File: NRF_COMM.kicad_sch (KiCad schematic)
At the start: 2 parts, among them U5 NRF24L01_Breakout

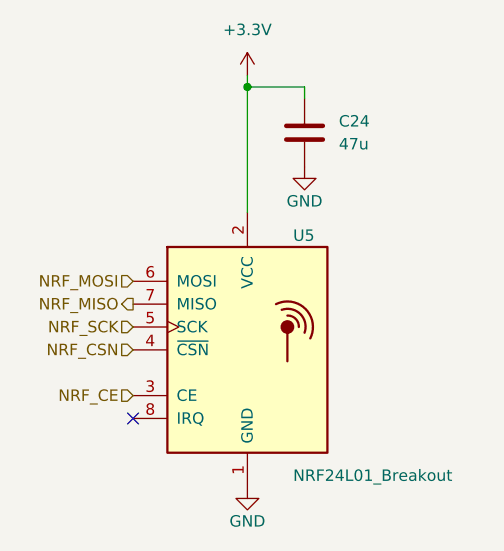
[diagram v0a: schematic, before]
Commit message: changed pins
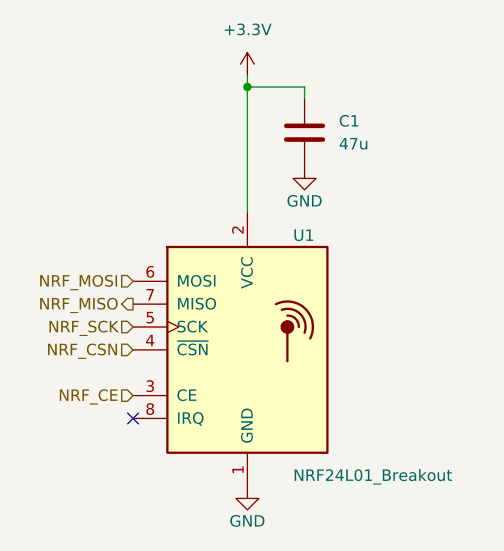
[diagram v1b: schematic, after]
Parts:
- C1: renamed from C24; footprint Capacitor_THT:CP_Radial_D5.0mm_P2.00mm -> Capacitor_THT:CP_Radial_D4.0mm_P1.50mm
- renumbered U5 to U1
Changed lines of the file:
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@@
   (symbol (lib_id "RF:NRF24L01_Breakout") (at 139.7 100.33 0) (unit 1)
     (in_bom yes) (on_board yes) (dnp no)
-    (property "Reference" "U5" (at 144.78 87.63 0)
+    (property "Reference" "U1" (at 144.78 87.63 0)
       (effects (font (size 1.27 1.27)) (justify left))
     )
@@
       (project "electrium-esc-v2"
         (path "/be00c12c-11fa-42cb-8a0b-46fcd24b2ced/81cbbca5-64b8-44af-87f0-aec946520ae6"
-          (reference "U5") (unit 1)
+          (reference "U1") (unit 1)
         )
       )
       (project "electrium-esc"
         (path "/d277d506-2f4d-497b-a498-1ff059e212d2/9d2b8e53-abda-48f4-a6e0-4b62c24d8218"
-          (reference "U?") (unit 1)
+          (reference "U5") (unit 1)
         )
       )
@@
   (symbol (lib_id "power:GND") (at 146.05 80.01 0) (unit 1)
     (in_bom yes) (on_board yes) (dnp no)
-    (property "Reference" "#PWR037" (at 146.05 86.36 0)
+    (property "Reference" "#PWR03" (at 146.05 86.36 0)
       (effects (font (size 1.27 1.27)) hide)
     )
@@
       (project "electrium-esc-v2"
         (path "/be00c12c-11fa-42cb-8a0b-46fcd24b2ced/81cbbca5-64b8-44af-87f0-aec946520ae6"
-          (reference "#PWR037") (unit 1)
+          (reference "#PWR03") (unit 1)
         )
       )
       (project "electrium-esc"
         (path "/d277d506-2f4d-497b-a498-1ff059e212d2/9d2b8e53-abda-48f4-a6e0-4b62c24d8218"
-          (reference "#PWR?") (unit 1)
+          (reference "#PWR072") (unit 1)
         )
       )
@@
   (symbol (lib_id "Device:C") (at 146.05 76.2 0) (unit 1)
     (in_bom yes) (on_board yes) (dnp no) (fields_autoplaced)
-    (property "Reference" "C24" (at 149.86 74.9299 0)
+    (property "Reference" "C1" (at 149.86 74.9299 0)
       (effects (font (size 1.27 1.27)) (justify left))
     )
@@
       (effects (font (size 1.27 1.27)) (justify left))
     )
-    (property "Footprint" "Capacitor_THT:CP_Radial_D5.0mm_P2.00mm" (at 147.0152 80.01 0)
+    (property "Footprint" "Capacitor_THT:CP_Radial_D4.0mm_P1.50mm" (at 147.0152 80.01 0)
       (effects (font (size 1.27 1.27)) hide)
     )
@@
       (project "electrium-esc-v2"
         (path "/be00c12c-11fa-42cb-8a0b-46fcd24b2ced/81cbbca5-64b8-44af-87f0-aec946520ae6"
-          (reference "C24") (unit 1)
+          (reference "C1") (unit 1)
         )
       )
       (project "electrium-esc"
         (path "/d277d506-2f4d-497b-a498-1ff059e212d2/9d2b8e53-abda-48f4-a6e0-4b62c24d8218"
-          (reference "C?") (unit 1)
+          (reference "C75") (unit 1)
         )
       )
@@
   (symbol (lib_id "power:+3.3V") (at 139.7 69.85 0) (unit 1)
     (in_bom yes) (on_board yes) (dnp no) (fields_autoplaced)
-    (property "Reference" "#PWR035" (at 139.7 73.66 0)
+    (property "Reference" "#PWR01" (at 139.7 73.66 0)
       (effects (font (size 1.27 1.27)) hide)
     )
@@
       (project "electrium-esc-v2"
         (path "/be00c12c-11fa-42cb-8a0b-46fcd24b2ced/81cbbca5-64b8-44af-87f0-aec946520ae6"
-          (reference "#PWR035") (unit 1)
+          (reference "#PWR01") (unit 1)
         )
       )
       (project "electrium-esc"
         (path "/d277d506-2f4d-497b-a498-1ff059e212d2/9d2b8e53-abda-48f4-a6e0-4b62c24d8218"
-          (reference "#PWR?") (unit 1)
+          (reference "#PWR071") (unit 1)
         )
       )
@@
   (symbol (lib_id "power:GND") (at 139.7 115.57 0) (unit 1)
     (in_bom yes) (on_board yes) (dnp no)
-    (property "Reference" "#PWR036" (at 139.7 121.92 0)
+    (property "Reference" "#PWR02" (at 139.7 121.92 0)
       (effects (font (size 1.27 1.27)) hide)
     )
@@
       (project "electrium-esc-v2"
         (path "/be00c12c-11fa-42cb-8a0b-46fcd24b2ced/81cbbca5-64b8-44af-87f0-aec946520ae6"
-          (reference "#PWR036") (unit 1)
+          (reference "#PWR02") (unit 1)
         )
       )
       (project "electrium-esc"
         (path "/d277d506-2f4d-497b-a498-1ff059e212d2/9d2b8e53-abda-48f4-a6e0-4b62c24d8218"
-          (reference "#PWR?") (unit 1)
+          (reference "#PWR073") (unit 1)
         )
       )

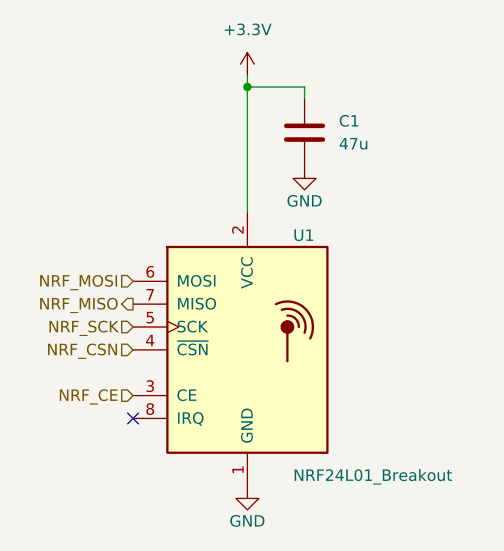
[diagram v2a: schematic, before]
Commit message: Add reference changes
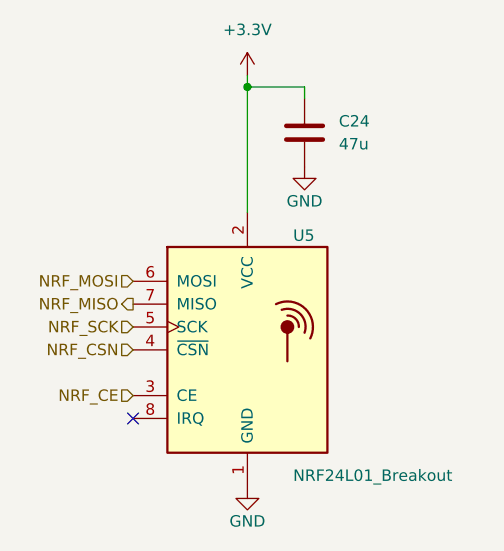
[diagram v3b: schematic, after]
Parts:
- C24: renamed from C1; footprint Capacitor_THT:CP_Radial_D4.0mm_P1.50mm -> Capacitor_THT:CP_Radial_D5.0mm_P2.00mm
- renumbered U1 to U5
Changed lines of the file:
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@@
   (symbol (lib_id "RF:NRF24L01_Breakout") (at 139.7 100.33 0) (unit 1)
     (in_bom yes) (on_board yes) (dnp no)
-    (property "Reference" "U1" (at 144.78 87.63 0)
+    (property "Reference" "U5" (at 144.78 87.63 0)
       (effects (font (size 1.27 1.27)) (justify left))
     )
@@
       (project "electrium-esc-v2"
         (path "/be00c12c-11fa-42cb-8a0b-46fcd24b2ced/81cbbca5-64b8-44af-87f0-aec946520ae6"
-          (reference "U1") (unit 1)
+          (reference "U5") (unit 1)
         )
       )
       (project "electrium-esc"
         (path "/d277d506-2f4d-497b-a498-1ff059e212d2/9d2b8e53-abda-48f4-a6e0-4b62c24d8218"
-          (reference "U5") (unit 1)
+          (reference "U?") (unit 1)
         )
       )
@@
   (symbol (lib_id "power:GND") (at 146.05 80.01 0) (unit 1)
     (in_bom yes) (on_board yes) (dnp no)
-    (property "Reference" "#PWR03" (at 146.05 86.36 0)
+    (property "Reference" "#PWR037" (at 146.05 86.36 0)
       (effects (font (size 1.27 1.27)) hide)
     )
@@
       (project "electrium-esc-v2"
         (path "/be00c12c-11fa-42cb-8a0b-46fcd24b2ced/81cbbca5-64b8-44af-87f0-aec946520ae6"
-          (reference "#PWR03") (unit 1)
+          (reference "#PWR037") (unit 1)
         )
       )
       (project "electrium-esc"
         (path "/d277d506-2f4d-497b-a498-1ff059e212d2/9d2b8e53-abda-48f4-a6e0-4b62c24d8218"
-          (reference "#PWR072") (unit 1)
+          (reference "#PWR?") (unit 1)
         )
       )
@@
   (symbol (lib_id "Device:C") (at 146.05 76.2 0) (unit 1)
     (in_bom yes) (on_board yes) (dnp no) (fields_autoplaced)
-    (property "Reference" "C1" (at 149.86 74.9299 0)
+    (property "Reference" "C24" (at 149.86 74.9299 0)
       (effects (font (size 1.27 1.27)) (justify left))
     )
@@
       (effects (font (size 1.27 1.27)) (justify left))
     )
-    (property "Footprint" "Capacitor_THT:CP_Radial_D4.0mm_P1.50mm" (at 147.0152 80.01 0)
+    (property "Footprint" "Capacitor_THT:CP_Radial_D5.0mm_P2.00mm" (at 147.0152 80.01 0)
       (effects (font (size 1.27 1.27)) hide)
     )
@@
       (project "electrium-esc-v2"
         (path "/be00c12c-11fa-42cb-8a0b-46fcd24b2ced/81cbbca5-64b8-44af-87f0-aec946520ae6"
-          (reference "C1") (unit 1)
+          (reference "C24") (unit 1)
         )
       )
       (project "electrium-esc"
         (path "/d277d506-2f4d-497b-a498-1ff059e212d2/9d2b8e53-abda-48f4-a6e0-4b62c24d8218"
-          (reference "C75") (unit 1)
+          (reference "C?") (unit 1)
         )
       )
@@
   (symbol (lib_id "power:+3.3V") (at 139.7 69.85 0) (unit 1)
     (in_bom yes) (on_board yes) (dnp no) (fields_autoplaced)
-    (property "Reference" "#PWR01" (at 139.7 73.66 0)
+    (property "Reference" "#PWR035" (at 139.7 73.66 0)
       (effects (font (size 1.27 1.27)) hide)
     )
@@
       (project "electrium-esc-v2"
         (path "/be00c12c-11fa-42cb-8a0b-46fcd24b2ced/81cbbca5-64b8-44af-87f0-aec946520ae6"
-          (reference "#PWR01") (unit 1)
+          (reference "#PWR035") (unit 1)
         )
       )
       (project "electrium-esc"
         (path "/d277d506-2f4d-497b-a498-1ff059e212d2/9d2b8e53-abda-48f4-a6e0-4b62c24d8218"
-          (reference "#PWR071") (unit 1)
+          (reference "#PWR?") (unit 1)
         )
       )
@@
   (symbol (lib_id "power:GND") (at 139.7 115.57 0) (unit 1)
     (in_bom yes) (on_board yes) (dnp no)
-    (property "Reference" "#PWR02" (at 139.7 121.92 0)
+    (property "Reference" "#PWR036" (at 139.7 121.92 0)
       (effects (font (size 1.27 1.27)) hide)
     )
@@
       (project "electrium-esc-v2"
         (path "/be00c12c-11fa-42cb-8a0b-46fcd24b2ced/81cbbca5-64b8-44af-87f0-aec946520ae6"
-          (reference "#PWR02") (unit 1)
+          (reference "#PWR036") (unit 1)
         )
       )
       (project "electrium-esc"
         (path "/d277d506-2f4d-497b-a498-1ff059e212d2/9d2b8e53-abda-48f4-a6e0-4b62c24d8218"
-          (reference "#PWR073") (unit 1)
+          (reference "#PWR?") (unit 1)
         )
       )
